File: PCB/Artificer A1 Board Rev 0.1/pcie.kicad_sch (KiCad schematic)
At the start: 11 parts, among them U7 X3113WVS-36-9TV01

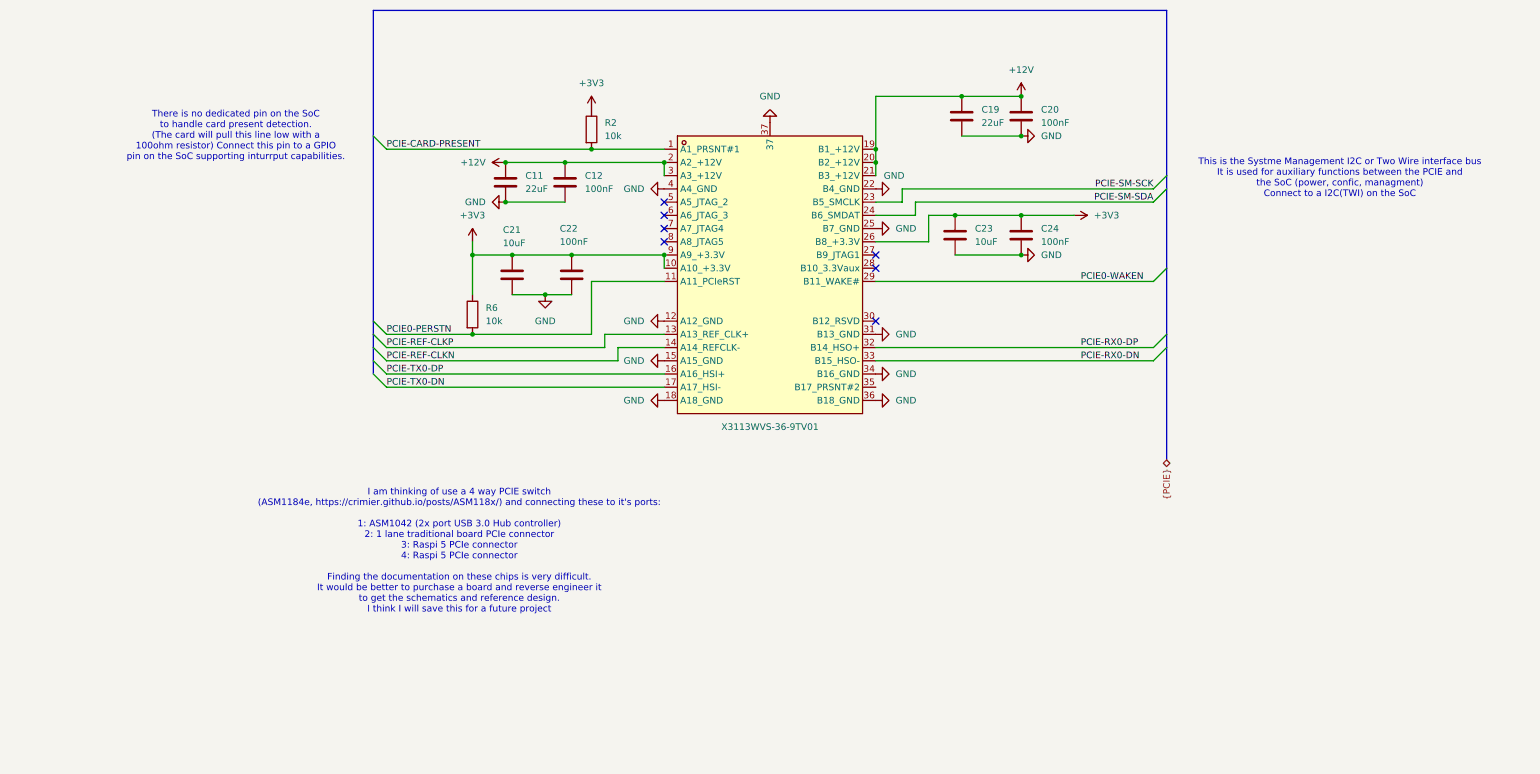
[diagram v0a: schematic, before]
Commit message: added features
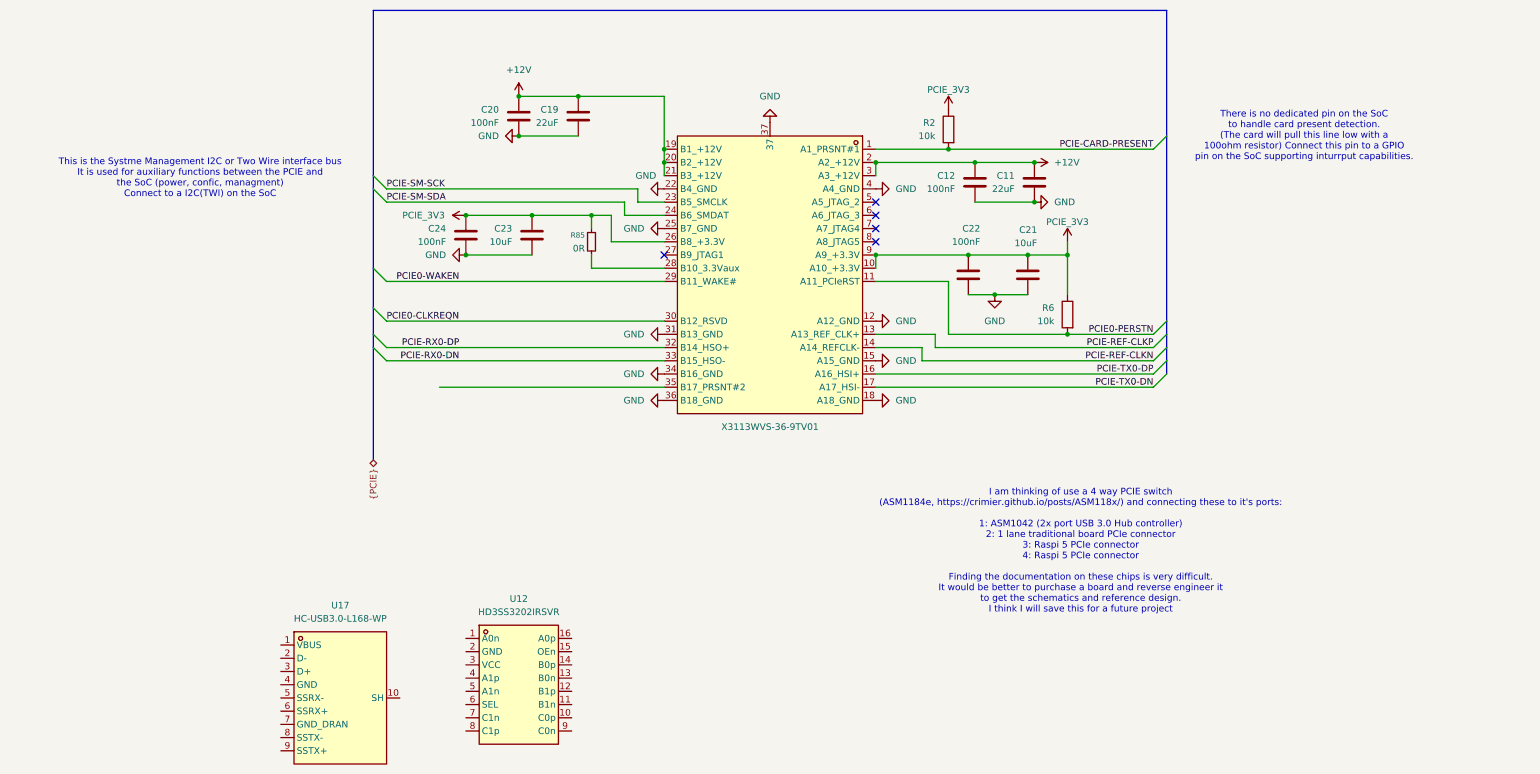
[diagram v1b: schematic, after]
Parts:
- added R85: 0R, symbol Device:R_Small
- added U12: HD3SS3202IRSVR, easyeda:UQFN-16_L2.6-W1.8-P0.40-BL, symbol easyeda:HD3SS3202IRSVR
- added U17: HC-USB3.0-L168-WP, easyeda:USB-TH_USB3.0-A, symbol easyeda:HC-USB3.0-L168-WP
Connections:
- net at U7.28 (B10_3.3Vaux): now also R85.2
- net PCIE0-CLKREQN: now reaches U7.30 (B12_RSVD)
- net +3V3 renamed PCIE_3V3
- net PCIE_3V3: now also R85.1
- no-connect marks 7 -> 5
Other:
- moved on the sheet: C11, C12, C19, C20, C21, C22, C23, C24, R2, R6
